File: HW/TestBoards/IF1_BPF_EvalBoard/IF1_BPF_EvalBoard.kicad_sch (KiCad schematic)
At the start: 8 parts, among them J1 SMA, J2 SMA, J3 SMA, J4 SMA

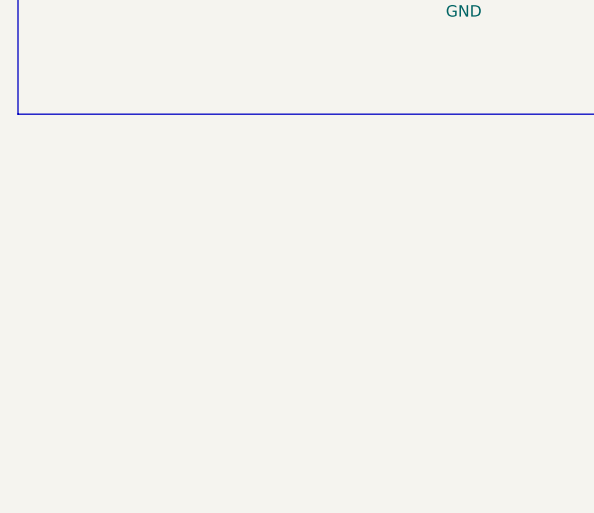
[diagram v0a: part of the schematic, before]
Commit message: LO1 Eval Board
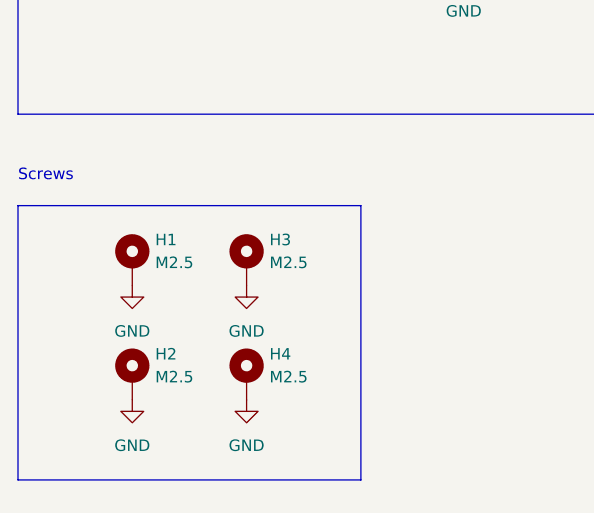
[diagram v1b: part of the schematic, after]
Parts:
- added H1, H2, H3, H4: M2.5, MountingHole:MountingHole_2.7mm_M2.5_Pad, symbol Mechanical:MountingHole_Pad
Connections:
- net GND: now also H1.1, H2.1, H3.1, H4.1
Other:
- note added: "Screws"
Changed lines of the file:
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@@
+    (stroke (width 0) (type default) (color 0 0 0 0))
+  )
+  (polyline (pts (xy 80.01 158.75) (xy 80.01 189.23))
     (stroke (width 0) (type default) (color 0 0 0 0))
   )
@@
     (stroke (width 0) (type default) (color 0 0 0 0))
   )
+  (polyline (pts (xy 80.01 158.75) (xy 118.11 158.75))
+    (stroke (width 0) (type default) (color 0 0 0 0))
+  )
   (wire (pts (xy 196.85 68.58) (xy 173.99 68.58))
     (stroke (width 0) (type default) (color 0 0 0 0))
@@
     (stroke (width 0) (type default) (color 0 0 0 0))
   )
+  (polyline (pts (xy 80.01 189.23) (xy 118.11 189.23))
+    (stroke (width 0) (type default) (color 0 0 0 0))
+  )
   (polyline (pts (xy 219.71 148.59) (xy 219.71 104.14))
     (stroke (width 0) (type default) (color 0 0 0 0))
@@
     (stroke (width 0) (type default) (color 0 0 0 0))
   )
+  (polyline (pts (xy 118.11 189.23) (xy 118.11 158.75))
+    (stroke (width 0) (type default) (color 0 0 0 0))
+  )
   (wire (pts (xy 157.48 77.47) (xy 157.48 80.01))
     (stroke (width 0) (type default) (color 0 0 0 0))
@@
     (effects (font (size 1.27 1.27)) (justify left bottom))
   )
+  (text "Screws" (at 80.01 156.21 0)
+    (effects (font (size 1.27 1.27)) (justify left bottom))
+  )
   (label "HPF_out2" (at 143.51 121.92 0)
     (effects (font (size 1.27 1.27)) (justify left bottom))
@@
   (label "RF_Out1" (at 187.96 68.58 0)
     (effects (font (size 1.27 1.27)) (justify left bottom))
+  )
+  (symbol (lib_id "Mechanical:MountingHole_Pad") (at 92.71 177.8 0) (unit 1)
+    (in_bom yes) (on_board yes) (fields_autoplaced)
+    (property "Reference" "H2" (id 0) (at 95.25 175.2599 0)
+      (effects (font (size 1.27 1.27)) (justify left))
+    )
+    (property "Value" "M2.5" (id 1) (at 95.25 177.7999 0)
+      (effects (font (size 1.27 1.27)) (justify left))
+    )
+    (property "Footprint" "MountingHole:MountingHole_2.7mm_M2.5_Pad" (id 2) (at 92.71 177.8 0)
+      (effects (font (size 1.27 1.27)) hide)
+    )
+    (property "Datasheet" "~" (id 3) (at 92.71 177.8 0)
+      (effects (font (size 1.27 1.27)) hide)
+    )
+    (pin "1")
+  )
+  (symbol (lib_id "power:GND") (at 105.41 180.34 0) (mirror y) (unit 1)
+    (in_bom yes) (on_board yes) (fields_autoplaced)
+    (property "Reference" "#PWR09" (id 0) (at 105.41 186.69 0)
+      (effects (font (size 1.27 1.27)) hide)
+    )
+    (property "Value" "GND" (id 1) (at 105.41 185.42 0))
+    (property "Footprint" "" (id 2) (at 105.41 180.34 0)
+      (effects (font (size 1.27 1.27)) hide)
+    )
+    (property "Datasheet" "" (id 3) (at 105.41 180.34 0)
+      (effects (font (size 1.27 1.27)) hide)
+    )
+    (pin "1")
+  )
+  (symbol (lib_id "Mechanical:MountingHole_Pad") (at 105.41 165.1 0) (unit 1)
+    (in_bom yes) (on_board yes) (fields_autoplaced)
+    (property "Reference" "H3" (id 0) (at 107.95 162.5599 0)
+      (effects (font (size 1.27 1.27)) (justify left))
+    )
+    (property "Value" "M2.5" (id 1) (at 107.95 165.0999 0)
+      (effects (font (size 1.27 1.27)) (justify left))
+    )
+    (property "Footprint" "MountingHole:MountingHole_2.7mm_M2.5_Pad" (id 2) (at 105.41 165.1 0)
+      (effects (font (size 1.27 1.27)) hide)
+    )
+    (property "Datasheet" "~" (id 3) (at 105.41 165.1 0)
+      (effects (font (size 1.27 1.27)) hide)
+    )
+    (pin "1")
   )
   (symbol (lib_id "power:GND") (at 173.99 82.55 0) (mirror y) (unit 1)
@@
     (pin "1")
   )
+  (symbol (lib_id "power:GND") (at 92.71 167.64 0) (mirror y) (unit 1)
+    (in_bom yes) (on_board yes) (fields_autoplaced)
+    (property "Reference" "#PWR06" (id 0) (at 92.71 173.99 0)
+      (effects (font (size 1.27 1.27)) hide)
+    )
+    (property "Value" "GND" (id 1) (at 92.71 172.72 0))
+    (property "Footprint" "" (id 2) (at 92.71 167.64 0)
+      (effects (font (size 1.27 1.27)) hide)
+    )
+    (property "Datasheet" "" (id 3) (at 92.71 167.64 0)
+      (effects (font (size 1.27 1.27)) hide)
+    )
+    (pin "1")
+  )
   (symbol (lib_id "power:GND") (at 129.54 78.74 0) (mirror y) (unit 1)
     (in_bom yes) (on_board yes) (fields_autoplaced)
@@
     )
     (property "Datasheet" "" (id 3) (at 199.39 73.66 0)
+      (effects (font (size 1.27 1.27)) hide)
+    )
+    (pin "1")
+  )
+  (symbol (lib_id "Mechanical:MountingHole_Pad") (at 92.71 165.1 0) (unit 1)
+    (in_bom yes) (on_board yes) (fields_autoplaced)
+    (property "Reference" "H1" (id 0) (at 95.25 162.5599 0)
+      (effects (font (size 1.27 1.27)) (justify left))
+    )
+    (property "Value" "M2.5" (id 1) (at 95.25 165.0999 0)
+      (effects (font (size 1.27 1.27)) (justify left))
+    )
+    (property "Footprint" "MountingHole:MountingHole_2.7mm_M2.5_Pad" (id 2) (at 92.71 165.1 0)
+      (effects (font (size 1.27 1.27)) hide)
+    )
+    (property "Datasheet" "~" (id 3) (at 92.71 165.1 0)
       (effects (font (size 1.27 1.27)) hide)
     )
@@
     (pin "S4")
   )
+  (symbol (lib_id "power:GND") (at 92.71 180.34 0) (mirror y) (unit 1)
+    (in_bom yes) (on_board yes) (fields_autoplaced)
+    (property "Reference" "#PWR07" (id 0) (at 92.71 186.69 0)
+      (effects (font (size 1.27 1.27)) hide)
+    )
+    (property "Value" "GND" (id 1) (at 92.71 185.42 0))
+    (property "Footprint" "" (id 2) (at 92.71 180.34 0)
+      (effects (font (size 1.27 1.27)) hide)
+    )
+    (property "Datasheet" "" (id 3) (at 92.71 180.34 0)
+      (effects (font (size 1.27 1.27)) hide)
+    )
+    (pin "1")
+  )
   (symbol (lib_id "power:GND") (at 166.37 87.63 0) (mirror y) (unit 1)
     (in_bom yes) (on_board yes) (fields_autoplaced)
@@
     )
     (property "Datasheet" "" (id 3) (at 157.48 125.73 0)
+      (effects (font (size 1.27 1.27)) hide)
+    )
+    (pin "1")
+  )
+  (symbol (lib_id "power:GND") (at 105.41 167.64 0) (mirror y) (unit 1)
+    (in_bom yes) (on_board yes) (fields_autoplaced)
+    (property "Reference" "#PWR08" (id 0) (at 105.41 173.99 0)
+      (effects (font (size 1.27 1.27)) hide)
+    )
+    (property "Value" "GND" (id 1) (at 105.41 172.72 0))
+    (property "Footprint" "" (id 2) (at 105.41 167.64 0)
+      (effects (font (size 1.27 1.27)) hide)
+    )
+    (property "Datasheet" "" (id 3) (at 105.41 167.64 0)
       (effects (font (size 1.27 1.27)) hide)
     )
@@
     (pin "4")
   )
+  (symbol (lib_id "Mechanical:MountingHole_Pad") (at 105.41 177.8 0) (unit 1)
+    (in_bom yes) (on_board yes) (fields_autoplaced)
+    (property "Reference" "H4" (id 0) (at 107.95 175.2599 0)
+      (effects (font (size 1.27 1.27)) (justify left))
+    )
+    (property "Value" "M2.5" (id 1) (at 107.95 177.7999 0)
+      (effects (font (size 1.27 1.27)) (justify left))
+    )
+    (property "Footprint" "MountingHole:MountingHole_2.7mm_M2.5_Pad" (id 2) (at 105.41 177.8 0)
+      (effects (font (size 1.27 1.27)) hide)
+    )
+    (property "Datasheet" "~" (id 3) (at 105.41 177.8 0)
+      (effects (font (size 1.27 1.27)) hide)
+    )
+    (pin "1")
+  )
   (sheet_instances
     (path "/" (page "1"))
@@
       (reference "#PWR05") (unit 1) (value "GND") (footprint "")
     )
+    (path "/553899fd-a0fc-46cf-a50b-1ae22742f6fb"
+      (reference "#PWR06") (unit 1) (value "GND") (footprint "")
+    )
+    (path "/a4ed4ab8-e645-4676-a4cd-70da244518c3"
+      (reference "#PWR07") (unit 1) (value "GND") (footprint "")
+    )
+    (path "/b401dd2f-1227-4907-9a24-58317335779e"
+      (reference "#PWR08") (unit 1) (value "GND") (footprint "")
+    )
+    (path "/1a3f0467-fc30-4ad9-abbb-e48a93a263a1"
+      (reference "#PWR09") (unit 1) (value "GND") (footprint "")
+    )
     (path "/68740b93-1535-40d7-bf59-ab923bf0b45d"
       (reference "#PWR0101") (unit 1) (value "GND") (footprint "")
@@
       (reference "FL4") (unit 1) (value "LFCW-8000+") (footprint "GGS_RF:JC0603C-1")
     )
+    (path "/6a18938a-7549-4433-9522-e0a35d59b2d3"
+      (reference "H1") (unit 1) (value "M2.5") (footprint "MountingHole:MountingHole_2.7mm_M2.5_Pad")
+    )
+    (path "/0806c0e7-f097-4b0f-b043-e2459aee844e"
+      (reference "H2") (unit 1) (value "M2.5") (footprint "MountingHole:MountingHole_2.7mm_M2.5_Pad")
+    )
+    (path "/1b2c45a1-b01e-4698-862d-446b1e1278aa"
+      (reference "H3") (unit 1) (value "M2.5") (footprint "MountingHole:MountingHole_2.7mm_M2.5_Pad")
+    )
+    (path "/f22ea2ac-090d-461b-81b4-2959d3962461"
+      (reference "H4") (unit 1) (value "M2.5") (footprint "MountingHole:MountingHole_2.7mm_M2.5_Pad")
+    )
     (path "/99d6b312-1146-4ee0-a9f8-ba6a1b945991"

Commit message: Added Evaluation Boards for RO4003C 1.52 mm
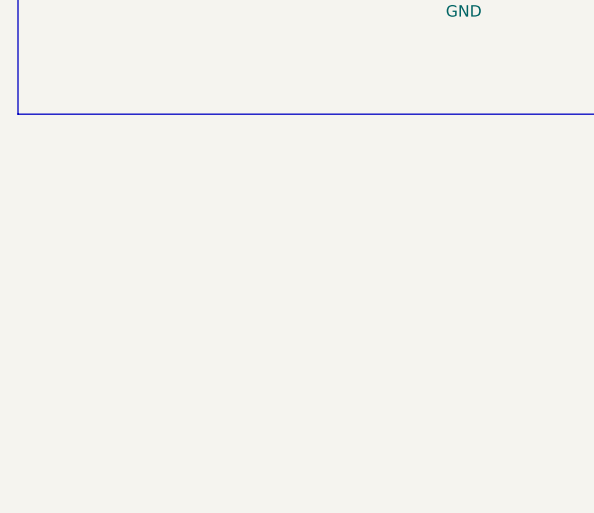
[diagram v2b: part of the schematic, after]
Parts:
- removed H1, H2, H3, H4: M2.5, MountingHole:MountingHole_2.7mm_M2.5_Pad, symbol Mechanical:MountingHole_Pad
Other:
- note removed: "Screws"
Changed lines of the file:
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@@
-    (stroke (width 0) (type default) (color 0 0 0 0))
-  )
-  (polyline (pts (xy 80.01 158.75) (xy 80.01 189.23))
     (stroke (width 0) (type default) (color 0 0 0 0))
   )
@@
     (stroke (width 0) (type default) (color 0 0 0 0))
   )
-  (polyline (pts (xy 80.01 158.75) (xy 118.11 158.75))
-    (stroke (width 0) (type default) (color 0 0 0 0))
-  )
   (wire (pts (xy 196.85 68.58) (xy 173.99 68.58))
     (stroke (width 0) (type default) (color 0 0 0 0))
@@
     (stroke (width 0) (type default) (color 0 0 0 0))
   )
-  (polyline (pts (xy 80.01 189.23) (xy 118.11 189.23))
-    (stroke (width 0) (type default) (color 0 0 0 0))
-  )
   (polyline (pts (xy 219.71 148.59) (xy 219.71 104.14))
     (stroke (width 0) (type default) (color 0 0 0 0))
@@
     (stroke (width 0) (type default) (color 0 0 0 0))
   )
-  (polyline (pts (xy 118.11 189.23) (xy 118.11 158.75))
-    (stroke (width 0) (type default) (color 0 0 0 0))
-  )
   (wire (pts (xy 157.48 77.47) (xy 157.48 80.01))
     (stroke (width 0) (type default) (color 0 0 0 0))
@@
     (effects (font (size 1.27 1.27)) (justify left bottom))
   )
-  (text "Screws" (at 80.01 156.21 0)
-    (effects (font (size 1.27 1.27)) (justify left bottom))
-  )
   (label "HPF_out2" (at 143.51 121.92 0)
     (effects (font (size 1.27 1.27)) (justify left bottom))
@@
   (label "RF_Out1" (at 187.96 68.58 0)
     (effects (font (size 1.27 1.27)) (justify left bottom))
-  )
-  (symbol (lib_id "Mechanical:MountingHole_Pad") (at 92.71 177.8 0) (unit 1)
-    (in_bom yes) (on_board yes) (fields_autoplaced)
-    (property "Reference" "H2" (id 0) (at 95.25 175.2599 0)
-      (effects (font (size 1.27 1.27)) (justify left))
-    )
-    (property "Value" "M2.5" (id 1) (at 95.25 177.7999 0)
-      (effects (font (size 1.27 1.27)) (justify left))
-    )
-    (property "Footprint" "MountingHole:MountingHole_2.7mm_M2.5_Pad" (id 2) (at 92.71 177.8 0)
-      (effects (font (size 1.27 1.27)) hide)
-    )
-    (property "Datasheet" "~" (id 3) (at 92.71 177.8 0)
-      (effects (font (size 1.27 1.27)) hide)
-    )
-    (pin "1")
-  )
-  (symbol (lib_id "power:GND") (at 105.41 180.34 0) (mirror y) (unit 1)
-    (in_bom yes) (on_board yes) (fields_autoplaced)
-    (property "Reference" "#PWR09" (id 0) (at 105.41 186.69 0)
-      (effects (font (size 1.27 1.27)) hide)
-    )
-    (property "Value" "GND" (id 1) (at 105.41 185.42 0))
-    (property "Footprint" "" (id 2) (at 105.41 180.34 0)
-      (effects (font (size 1.27 1.27)) hide)
-    )
-    (property "Datasheet" "" (id 3) (at 105.41 180.34 0)
-      (effects (font (size 1.27 1.27)) hide)
-    )
-    (pin "1")
-  )
-  (symbol (lib_id "Mechanical:MountingHole_Pad") (at 105.41 165.1 0) (unit 1)
-    (in_bom yes) (on_board yes) (fields_autoplaced)
-    (property "Reference" "H3" (id 0) (at 107.95 162.5599 0)
-      (effects (font (size 1.27 1.27)) (justify left))
-    )
-    (property "Value" "M2.5" (id 1) (at 107.95 165.0999 0)
-      (effects (font (size 1.27 1.27)) (justify left))
-    )
-    (property "Footprint" "MountingHole:MountingHole_2.7mm_M2.5_Pad" (id 2) (at 105.41 165.1 0)
-      (effects (font (size 1.27 1.27)) hide)
-    )
-    (property "Datasheet" "~" (id 3) (at 105.41 165.1 0)
-      (effects (font (size 1.27 1.27)) hide)
-    )
-    (pin "1")
   )
   (symbol (lib_id "power:GND") (at 173.99 82.55 0) (mirror y) (unit 1)
@@
     (pin "1")
   )
-  (symbol (lib_id "power:GND") (at 92.71 167.64 0) (mirror y) (unit 1)
-    (in_bom yes) (on_board yes) (fields_autoplaced)
-    (property "Reference" "#PWR06" (id 0) (at 92.71 173.99 0)
-      (effects (font (size 1.27 1.27)) hide)
-    )
-    (property "Value" "GND" (id 1) (at 92.71 172.72 0))
-    (property "Footprint" "" (id 2) (at 92.71 167.64 0)
-      (effects (font (size 1.27 1.27)) hide)
-    )
-    (property "Datasheet" "" (id 3) (at 92.71 167.64 0)
-      (effects (font (size 1.27 1.27)) hide)
-    )
-    (pin "1")
-  )
   (symbol (lib_id "power:GND") (at 129.54 78.74 0) (mirror y) (unit 1)
     (in_bom yes) (on_board yes) (fields_autoplaced)
@@
     )
     (property "Datasheet" "" (id 3) (at 199.39 73.66 0)
-      (effects (font (size 1.27 1.27)) hide)
-    )
-    (pin "1")
-  )
-  (symbol (lib_id "Mechanical:MountingHole_Pad") (at 92.71 165.1 0) (unit 1)
-    (in_bom yes) (on_board yes) (fields_autoplaced)
-    (property "Reference" "H1" (id 0) (at 95.25 162.5599 0)
-      (effects (font (size 1.27 1.27)) (justify left))
-    )
-    (property "Value" "M2.5" (id 1) (at 95.25 165.0999 0)
-      (effects (font (size 1.27 1.27)) (justify left))
-    )
-    (property "Footprint" "MountingHole:MountingHole_2.7mm_M2.5_Pad" (id 2) (at 92.71 165.1 0)
-      (effects (font (size 1.27 1.27)) hide)
-    )
-    (property "Datasheet" "~" (id 3) (at 92.71 165.1 0)
       (effects (font (size 1.27 1.27)) hide)
     )
@@
     (pin "S4")
   )
-  (symbol (lib_id "power:GND") (at 92.71 180.34 0) (mirror y) (unit 1)
-    (in_bom yes) (on_board yes) (fields_autoplaced)
-    (property "Reference" "#PWR07" (id 0) (at 92.71 186.69 0)
-      (effects (font (size 1.27 1.27)) hide)
-    )
-    (property "Value" "GND" (id 1) (at 92.71 185.42 0))
-    (property "Footprint" "" (id 2) (at 92.71 180.34 0)
-      (effects (font (size 1.27 1.27)) hide)
-    )
-    (property "Datasheet" "" (id 3) (at 92.71 180.34 0)
-      (effects (font (size 1.27 1.27)) hide)
-    )
-    (pin "1")
-  )
   (symbol (lib_id "power:GND") (at 166.37 87.63 0) (mirror y) (unit 1)
     (in_bom yes) (on_board yes) (fields_autoplaced)
@@
     )
     (property "Datasheet" "" (id 3) (at 157.48 125.73 0)
-      (effects (font (size 1.27 1.27)) hide)
-    )
-    (pin "1")
-  )
-  (symbol (lib_id "power:GND") (at 105.41 167.64 0) (mirror y) (unit 1)
-    (in_bom yes) (on_board yes) (fields_autoplaced)
-    (property "Reference" "#PWR08" (id 0) (at 105.41 173.99 0)
-      (effects (font (size 1.27 1.27)) hide)
-    )
-    (property "Value" "GND" (id 1) (at 105.41 172.72 0))
-    (property "Footprint" "" (id 2) (at 105.41 167.64 0)
-      (effects (font (size 1.27 1.27)) hide)
-    )
-    (property "Datasheet" "" (id 3) (at 105.41 167.64 0)
       (effects (font (size 1.27 1.27)) hide)
     )
@@
     (pin "4")
   )
-  (symbol (lib_id "Mechanical:MountingHole_Pad") (at 105.41 177.8 0) (unit 1)
-    (in_bom yes) (on_board yes) (fields_autoplaced)
-    (property "Reference" "H4" (id 0) (at 107.95 175.2599 0)
-      (effects (font (size 1.27 1.27)) (justify left))
-    )
-    (property "Value" "M2.5" (id 1) (at 107.95 177.7999 0)
-      (effects (font (size 1.27 1.27)) (justify left))
-    )
-    (property "Footprint" "MountingHole:MountingHole_2.7mm_M2.5_Pad" (id 2) (at 105.41 177.8 0)
-      (effects (font (size 1.27 1.27)) hide)
-    )
-    (property "Datasheet" "~" (id 3) (at 105.41 177.8 0)
-      (effects (font (size 1.27 1.27)) hide)
-    )
-    (pin "1")
-  )
   (sheet_instances
     (path "/" (page "1"))
@@
       (reference "#PWR05") (unit 1) (value "GND") (footprint "")
     )
-    (path "/553899fd-a0fc-46cf-a50b-1ae22742f6fb"
-      (reference "#PWR06") (unit 1) (value "GND") (footprint "")
-    )
-    (path "/a4ed4ab8-e645-4676-a4cd-70da244518c3"
-      (reference "#PWR07") (unit 1) (value "GND") (footprint "")
-    )
-    (path "/b401dd2f-1227-4907-9a24-58317335779e"
-      (reference "#PWR08") (unit 1) (value "GND") (footprint "")
-    )
-    (path "/1a3f0467-fc30-4ad9-abbb-e48a93a263a1"
-      (reference "#PWR09") (unit 1) (value "GND") (footprint "")
-    )
     (path "/68740b93-1535-40d7-bf59-ab923bf0b45d"
       (reference "#PWR0101") (unit 1) (value "GND") (footprint "")
@@
       (reference "FL4") (unit 1) (value "LFCW-8000+") (footprint "GGS_RF:JC0603C-1")
     )
-    (path "/6a18938a-7549-4433-9522-e0a35d59b2d3"
-      (reference "H1") (unit 1) (value "M2.5") (footprint "MountingHole:MountingHole_2.7mm_M2.5_Pad")
-    )
-    (path "/0806c0e7-f097-4b0f-b043-e2459aee844e"
-      (reference "H2") (unit 1) (value "M2.5") (footprint "MountingHole:MountingHole_2.7mm_M2.5_Pad")
-    )
-    (path "/1b2c45a1-b01e-4698-862d-446b1e1278aa"
-      (reference "H3") (unit 1) (value "M2.5") (footprint "MountingHole:MountingHole_2.7mm_M2.5_Pad")
-    )
-    (path "/f22ea2ac-090d-461b-81b4-2959d3962461"
-      (reference "H4") (unit 1) (value "M2.5") (footprint "MountingHole:MountingHole_2.7mm_M2.5_Pad")
-    )
     (path "/99d6b312-1146-4ee0-a9f8-ba6a1b945991"
